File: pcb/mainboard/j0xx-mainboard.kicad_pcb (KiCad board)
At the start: 2 copper layers, 148 x 142 mm, 21 parts, among them J1 USB_C_Receptacle, Q1 BSS138, SW1 reset, U1 ATmega32U4-AU, Y1 Resonator

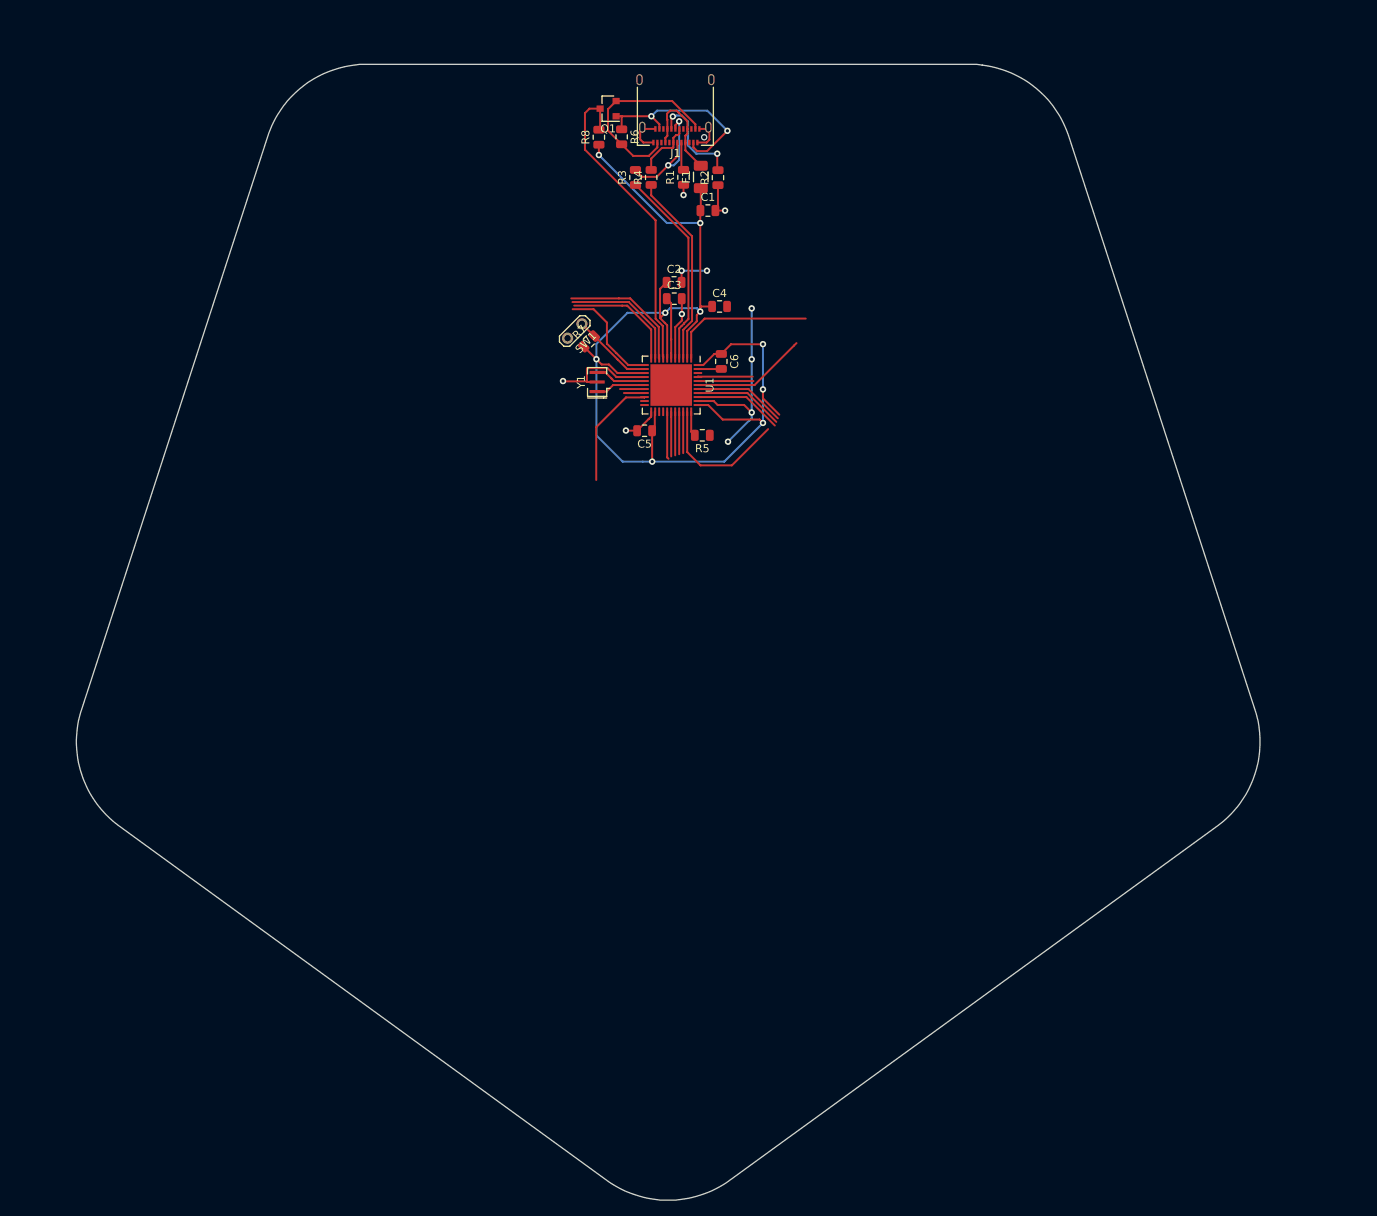
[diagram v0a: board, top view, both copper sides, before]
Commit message: wip
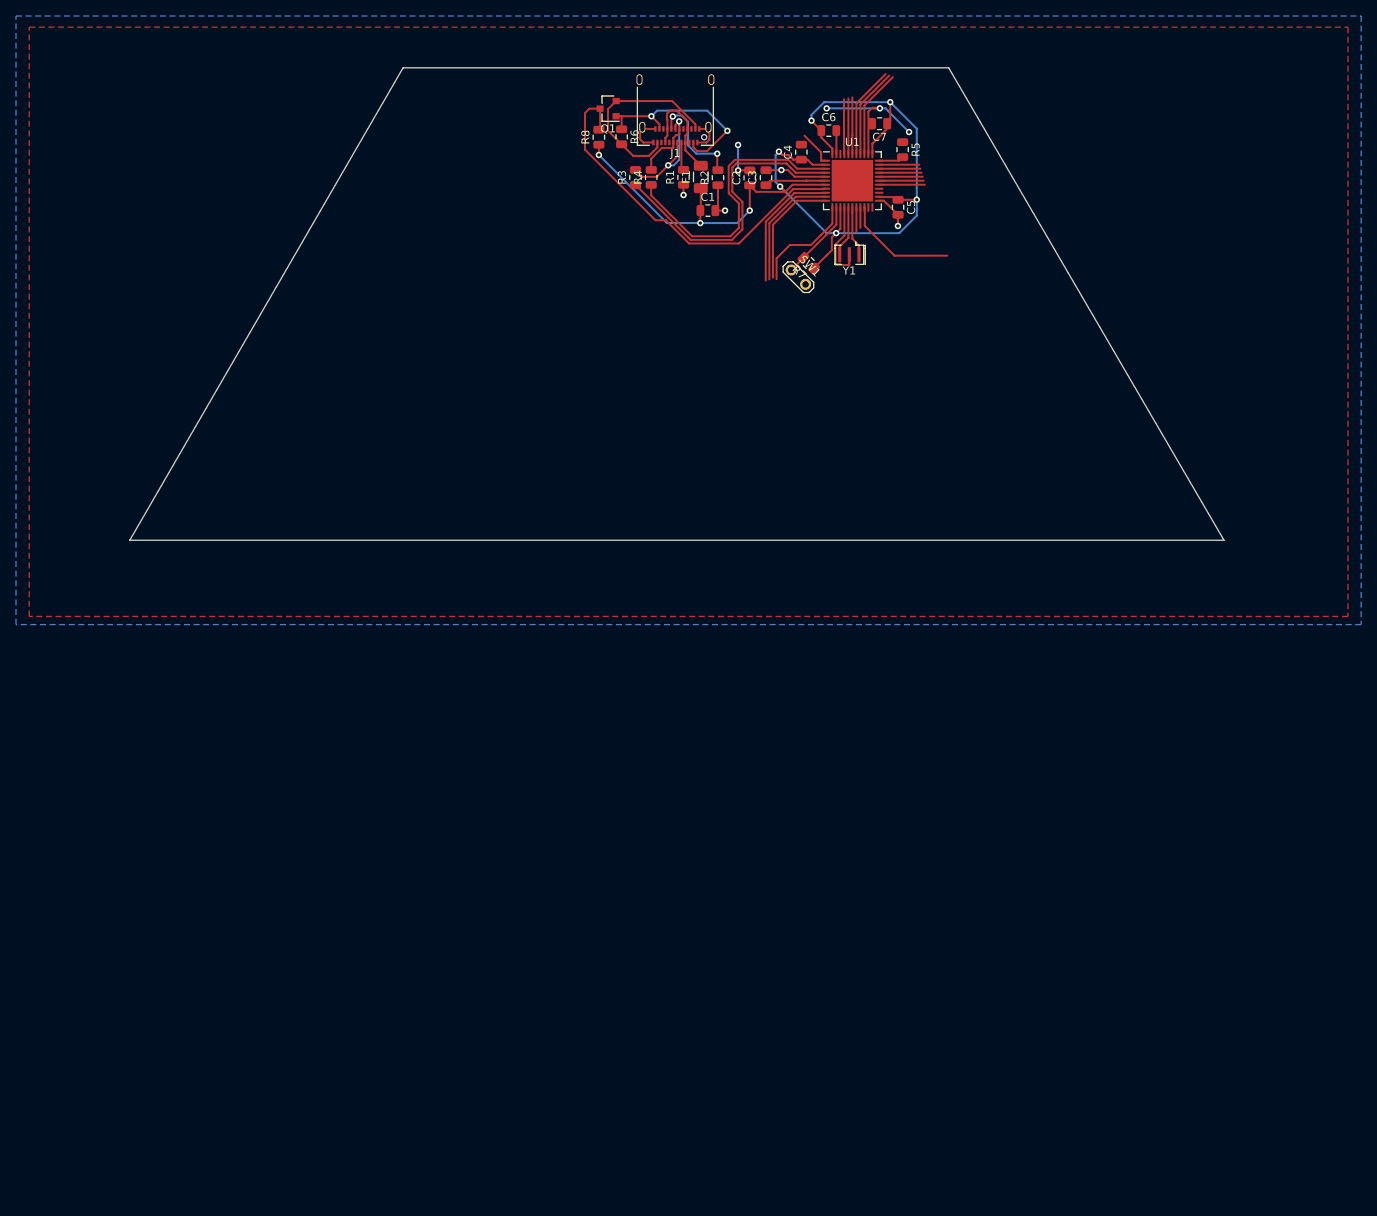
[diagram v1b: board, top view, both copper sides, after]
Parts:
- removed G***: LOGO, Outlines:pentagon
- added C7: 0.1u, Capacitor_SMD:C_0805_2012Metric, F.Cu at (237.4, 71.8)
- moved R5 43.6 mm to (240.2, 75.0), turned to 270 degrees
- moved C5 42.2 mm to (239.7, 82.2), turned to 270 degrees
- moved Y1 35.3 mm to (233.6, 88.1), turned to 180 degrees
- moved U1 34.1 mm to (234.0, 78.9), turned to 0 degrees
- moved C6 31.8 mm to (231.0, 72.6), turned to 0 degrees
- moved R7 29.2 mm to (228.5, 89.2), turned to 135 degrees
- moved SW1 27.0 mm to (226.3, 90.0), turned to 315 degrees
- moved C4 21.8 mm to (227.6, 75.3), turned to 90 degrees
- moved C3 19.0 mm to (223.2, 78.5), turned to 90 degrees
- moved C2 16.1 mm to (221.1, 78.5), turned to 90 degrees
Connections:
- J1 pad A10: (no net) -> Net-(J1-PadA10)
- J1 pad A3: (no net) -> Net-(J1-PadA3)
- J1 pad A8: (no net) -> Net-(J1-PadA8)
- J1 pad B10: (no net) -> Net-(J1-PadB10)
- J1 pad B3: (no net) -> Net-(J1-PadB3)
- J1 pad B8: (no net) -> Net-(J1-PadB8)
- U1 pad 1: (no net) -> BTN_MS
- U1 pad 10: (no net) -> BTN_LEFT
- U1 pad 11: (no net) -> BTN_DOWN
- U1 pad 12: (no net) -> BTN_RIGHT
- U1 pad 18: (no net) -> BTN_MODX
- U1 pad 19: (no net) -> BTN_MODY
- U1 pad 20: (no net) -> BTN_START
- U1 pad 21: (no net) -> Net-(U1-Pad21)
- U1 pad 22: (no net) -> Net-(U1-Pad22)
- U1 pad 25: (no net) -> Net-(U1-Pad25)
- U1 pad 26: (no net) -> Net-(U1-Pad26)
- U1 pad 27: (no net) -> BTN_CL
- U1 pad 28: (no net) -> BTN_CU
- U1 pad 29: (no net) -> BTN_CD
- U1 pad 30: (no net) -> BTN_A
- U1 pad 31: (no net) -> BTN_CR
- U1 pad 32: (no net) -> BTN_B
- U1 pad 36: (no net) -> BTN_X
- U1 pad 37: (no net) -> BTN_Z
- U1 pad 38: (no net) -> BTN_UP
- U1 pad 39: (no net) -> BTN_R
- U1 pad 40: (no net) -> BTN_Y
- U1 pad 41: (no net) -> BTN_LS
- U1 pad 42: (no net) -> Net-(U1-Pad42)
- U1 pad 9: (no net) -> BTN_L
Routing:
- net (no net): track 205.3 -> 0.00 mm
- net +5V: track 150.2 -> 128.2 mm
- net BTN_L: track 0.00 -> 16.4 mm
- net BTN_LEFT: track 0.00 -> 15.4 mm
- net BTN_DOWN: track 0.00 -> 14.5 mm
- net BTN_START: track 0.00 -> 14.2 mm
- net BTN_RIGHT: track 0.00 -> 13.4 mm
- net Net-(R3-Pad1): track 24.9 -> 37.4 mm
- net Net-(R4-Pad1): track 24.3 -> 36.0 mm
- net BTN_UP: track 0.00 -> 11.5 mm
- net BTN_Z: track 0.00 -> 11.3 mm
- net BTN_X: track 0.00 -> 11.1 mm
- net GND: track 74.3 -> 64.6 mm, vias 11 -> 9
- net GCCD5v: track 39.5 -> 47.2 mm
- net BTN_R: track 0.00 -> 7.08 mm
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- added copper zone on B.Cu, net GND
- added copper zone on F.Cu, net GND
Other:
- board size 148 x 142 mm -> 136.8 x 59.1 mm
